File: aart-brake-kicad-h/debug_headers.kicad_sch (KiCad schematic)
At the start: 0 parts

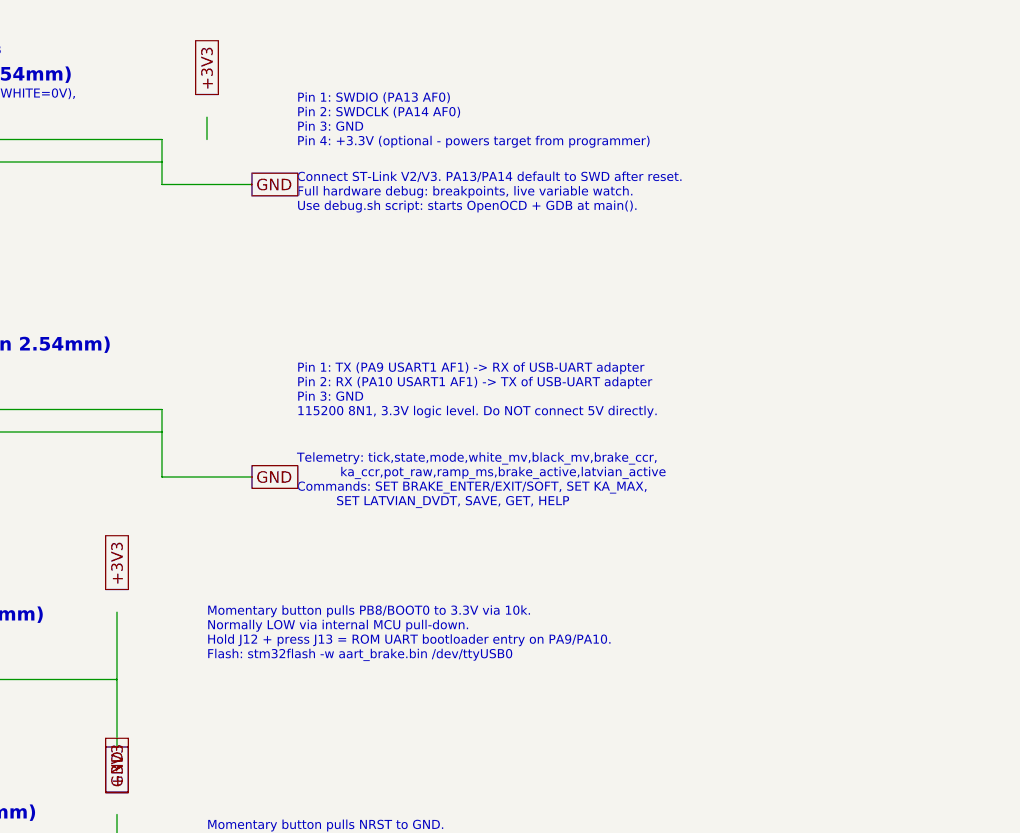
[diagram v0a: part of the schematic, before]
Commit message: Latest
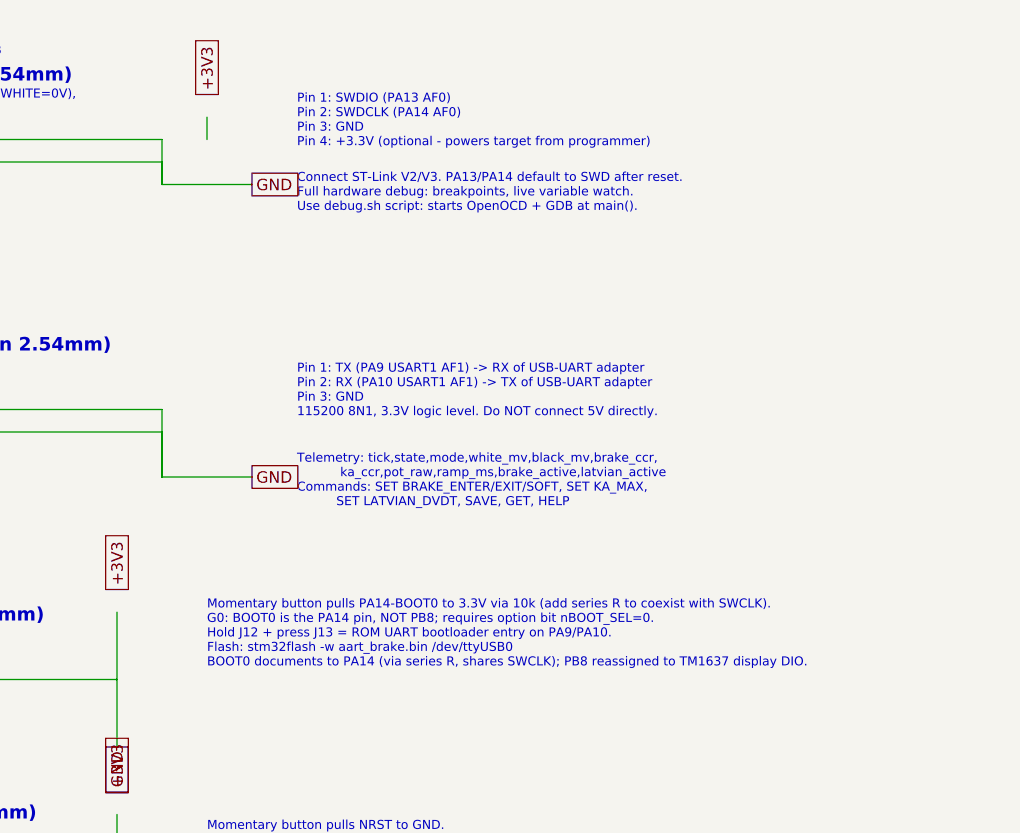
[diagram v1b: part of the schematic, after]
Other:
- note added: "Momentary button pulls PA14-BOOT0 to 3.3V via 10k (add series R to coexist with SWCLK). G0: BOOT0 is the PA14 pin, NOT PB8; requires option bit nBOOT_SEL=0. Hold J12 + press J13 = ROM UART bootloader entry on PA9/PA10. Flash: stm32flash -w aart_brake.bin /dev/ttyUSB0 BOOT0 documents to PA14 (via series R, shares SWCLK); PB8 reassigned to TM1637 display DIO."
- note removed: "Momentary button pulls PB8/BOOT0 to 3.3V via 10k. Normally LOW via internal MCU pull-down. Hold J12 + press J13 = ROM UART bootloader entry on PA9/PA10. Flash: stm32flash -w aart_brake.bin /dev/ttyUSB0"
